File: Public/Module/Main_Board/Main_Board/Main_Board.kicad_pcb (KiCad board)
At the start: 2 copper layers, 4 parts, among them J1 Conn_02x28_Odd_Even, J2 Conn_02x28_Odd_Even, J3 Conn_02x28_Odd_Even, J4 Conn_02x28_Odd_Even

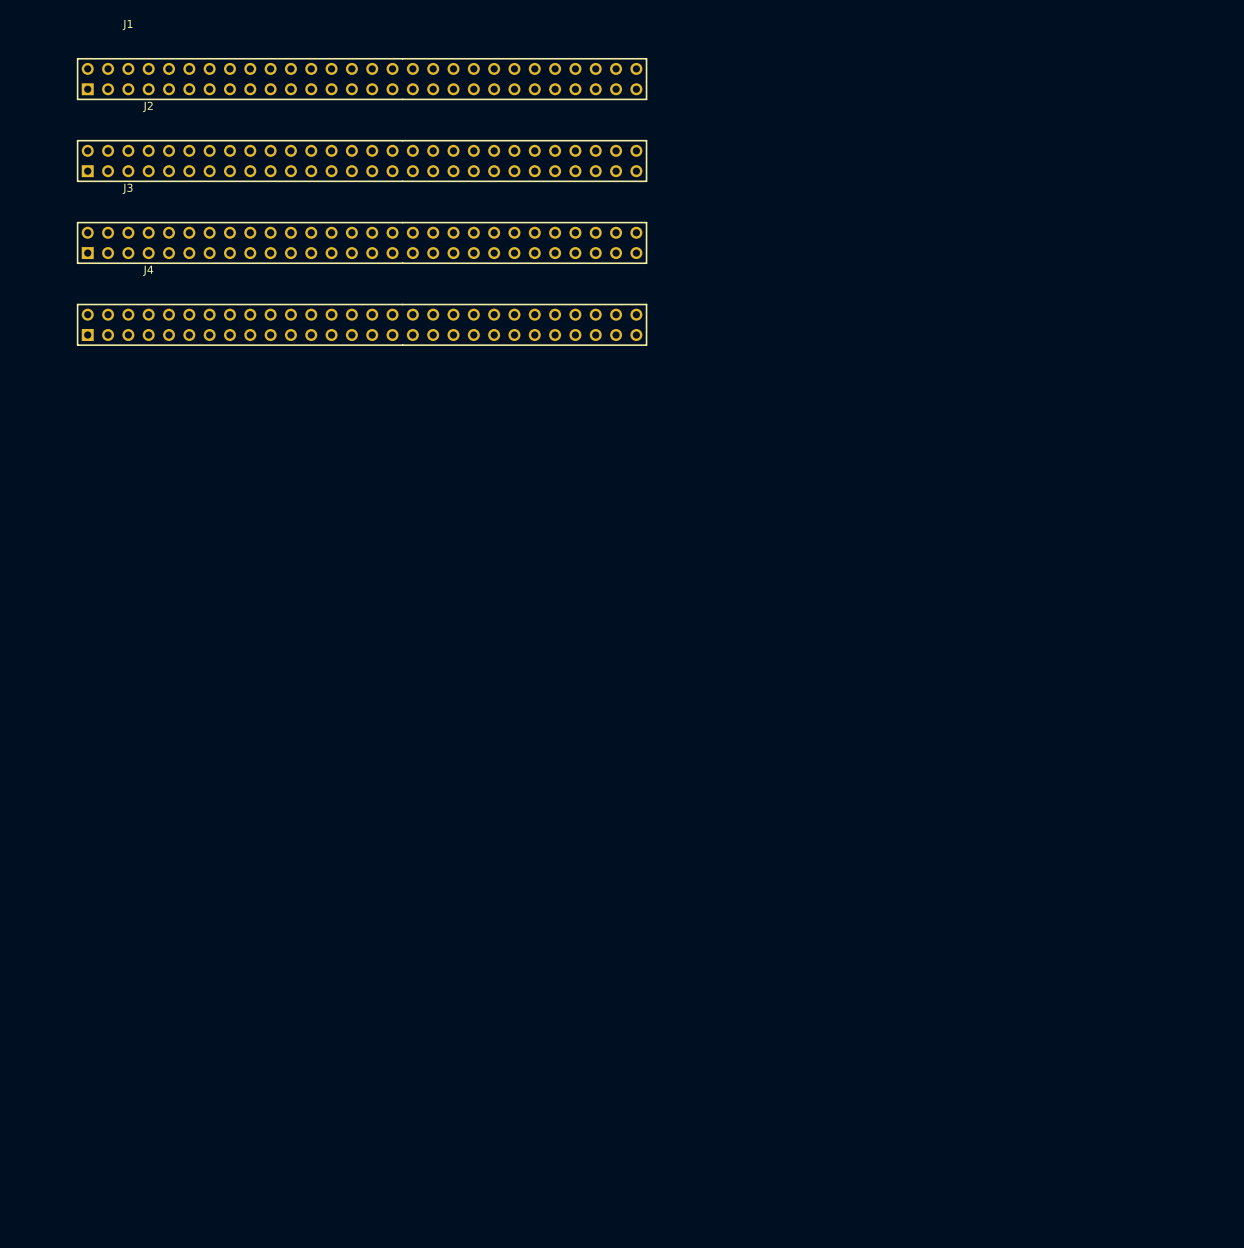
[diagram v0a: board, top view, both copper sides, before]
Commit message: 主板PCB绘制
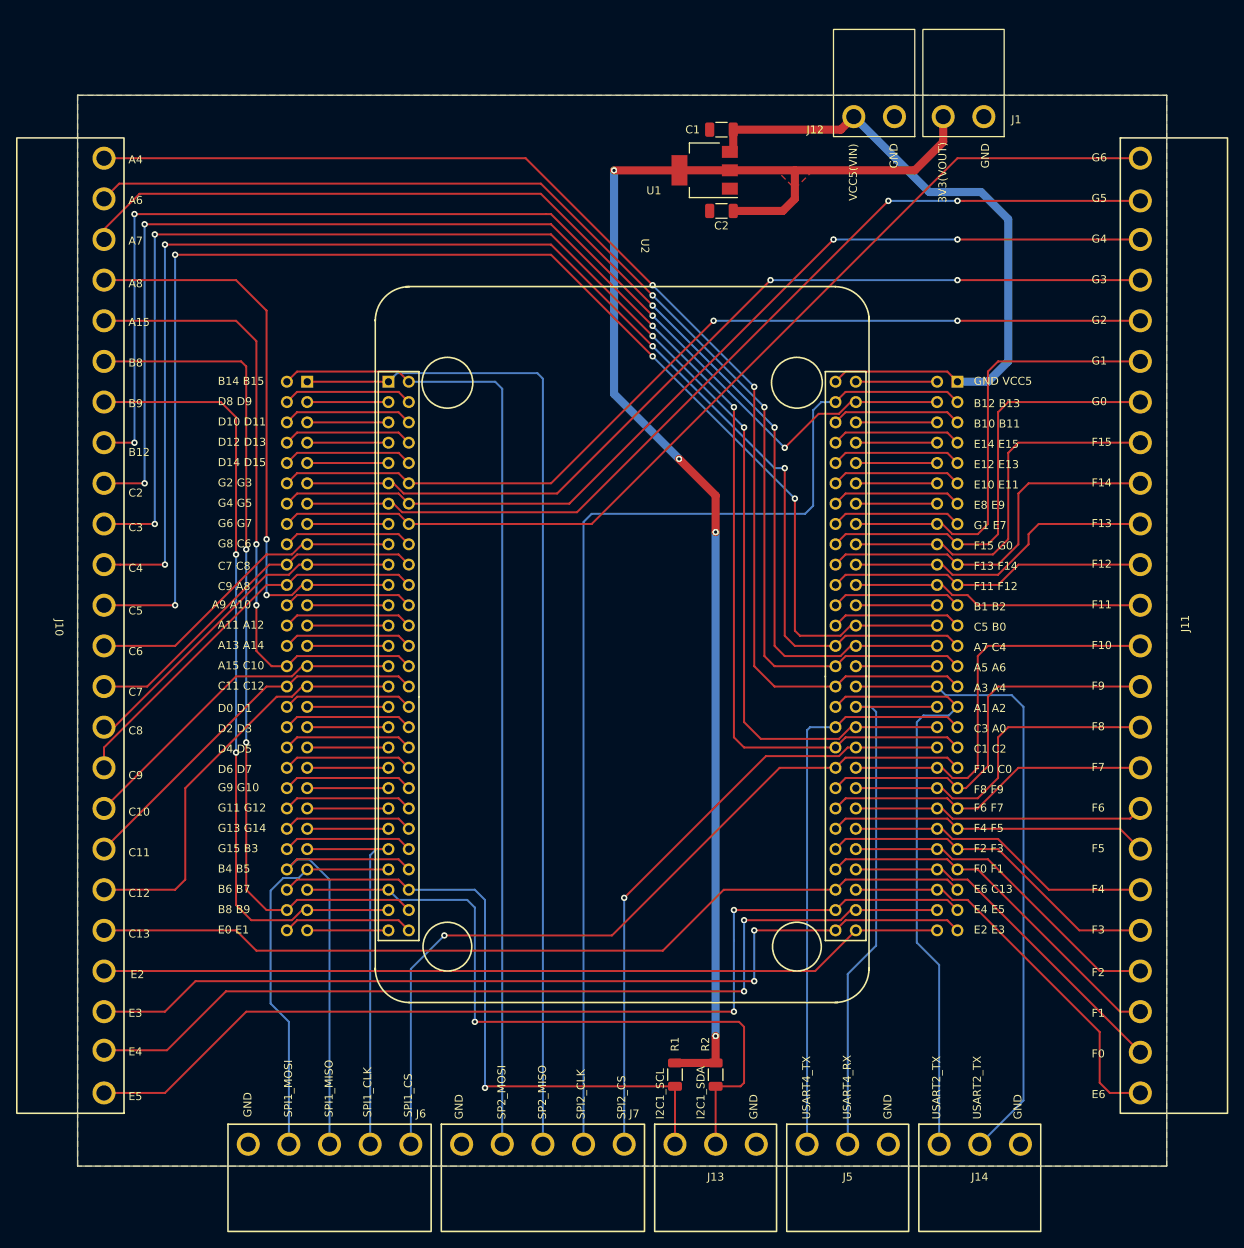
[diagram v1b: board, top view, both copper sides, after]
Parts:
- removed J2: Conn_02x28_Odd_Even, NEUDC:MCU_left
- added C1: 10uF, Capacitor_SMD:C_1206_3216Metric, F.Cu at (112.7, 42.1)
- added C2: 10uF, Capacitor_SMD:C_1206_3216Metric, F.Cu at (112.7, 52.3)
- added J10: Conn_01x24, NEUDC:Con_1_24, F.Cu at (35.6, 104.1)
- added J11: Conn_01x24, NEUDC:Con_1_24, F.Cu at (165.1, 104.1)
- added J12: Conn_01x02, NEUDC:Con_1_2, F.Cu at (131.8, 40.5)
- added J13: Conn_01x03, NEUDC:Con_1_3, F.Cu at (112.0, 169.0)
- added J14: Conn_01x03, NEUDC:Con_1_3, F.Cu at (145.0, 169.0)
- added J5: Conn_01x03, NEUDC:Con_1_3, F.Cu at (128.5, 169.0)
- added J6: Conn_01x05, NEUDC:Con_1_5, F.Cu at (63.8, 169.0)
- added J7: Conn_01x05, NEUDC:Con_1_5, F.Cu at (90.4, 169.0)
- added R1: 4.7k, Resistor_SMD:R_1206_3216Metric, F.Cu at (106.9, 160.3)
- added R2: 4.7k, Resistor_SMD:R_1206_3216Metric, F.Cu at (112.0, 160.3)
- added U1: LM1117MP-3.3, Package_TO_SOT_SMD:SOT-223-3_TabPin2, F.Cu at (110.6, 47.2)
- added U2: ~, NEUDC:qimin, F.Cu at (102.7, 56.7)
- J1: value Conn_02x28_Odd_Even -> Conn_01x02; footprint NEUDC:MCU_right -> NEUDC:Con_1_2
- J3, J4: moved to B.Cu
- moved J1 105.0 mm to (143.0, 40.5), turned to 180 degrees
- moved J3 100.2 mm to (134.6, 78.7), turned to -90 degrees
- moved J4 24.4 mm to (53.3, 81.3), turned to -90 degrees
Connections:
- J1 pad 1: /VCC5 -> GNDREF
- J1 pad 2: GNDREF -> /3V3
- J3 pad 3: /PB13 -> SPI2_CLK
- J3 pad 32: /PA3 -> USART2_RX
- J3 pad 33: /PA2 -> USART2_TX
- J3 pad 34: /PA1 -> USART4_RX
- J3 pad 35: /PA0 -> USART4_TX
- J3 pad 38: /PC1 -> SPI2_CS
- J3 pad 39: /PC0 -> SPI1_CS
- J4 pad 1: /PB14 -> SPI2_MISO
- J4 pad 2: /PB15 -> SPI2_MOSI
- J4 pad 47: /PB3 -> SPI1_CLK
- J4 pad 49: /PB5 -> SPI1_MOSI
- J4 pad 50: /PB4 -> SPI1_MISO
- J4 pad 51: /PB7 -> I2C1_SDA
- J4 pad 52: /PB6 -> I2C1_SCL
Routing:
- net /PC2: track 0.00 -> 191.4 mm, vias 0 -> 4
- net /PC3: track 0.00 -> 188.6 mm, vias 0 -> 4
- net /PC4: track 0.00 -> 180.8 mm, vias 0 -> 4
- net /3V3: track 0.00 -> 179.6 mm, vias 0 -> 4
- net /PC5: track 0.00 -> 177.9 mm, vias 0 -> 4
- net /PA4: track 0.00 -> 155.6 mm, vias 0 -> 2
- net /PA6: track 0.00 -> 151.7 mm, vias 0 -> 2
- net /PA7: track 0.00 -> 147.7 mm, vias 0 -> 2
- net /PB12: track 0.00 -> 147.2 mm, vias 0 -> 4
- net SPI2_CLK: track 0.00 -> 138.8 mm
- net /PG6: track 0.00 -> 126.7 mm
- net SPI2_MISO: track 0.00 -> 125.9 mm
- net /PE5: track 0.00 -> 124.7 mm, vias 0 -> 2
- net SPI2_MOSI: track 0.00 -> 122.8 mm
- net /PG4: track 0.00 -> 121.4 mm, vias 0 -> 2
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- added copper zone on F.Cu, net /3V3
- added copper zone on B.Cu, net GNDREF
- added copper zone on F.Cu, net GNDREF
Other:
- board outline added: 136.1 x 133.9 mm
- board text added: "3V3(VOUT)"
- board text added: "A1 A2"
- board text added: "A11 A12"
- board text added: "A13 A14"
- board text added: "A15"
- board text added: "A15 C10"
- board text added: "A3 A4"
- board text added: "A4"
- board text added: "A5 A6"
- board text added: "A6"
- board text added: "A7"
- board text added: "A7 C4"
- board text added: "A8"
- board text added: "A9 A10"
- board text added: "B1 B2"
- board text added: "B10 B11"
- board text added: "B12"
- board text added: "B12 B13"
- board text added: "B14 B15"
- board text added: "B4 B5"
- board text added: "B6 B7"
- board text added: "B8"
- board text added: "B8 B9"
- board text added: "B9"
- board text added: "C1 C2"
- board text added: "C10"
- board text added: "C11"
- board text added: "C11 C12"
- board text added: "C12"
- board text added: "C13"
- board text added: "C2"
- board text added: "C3"
- board text added: "C3 A0"
- board text added: "C4"
- board text added: "C5"
- board text added: "C5 B0"
- board text added: "C6"
- board text added: "C7"
- board text added: "C7 C8"
- board text added: "C8"
- board text added: "C9"
- board text added: "C9 A8"
- board text added: "D0 D1"
- board text added: "D10 D11"
- board text added: "D12 D13"
- board text added: "D14 D15"
- board text added: "D2 D3"
- board text added: "D4 D5"
- board text added: "D6 D7"
- board text added: "D8 D9"
- board text added: "E0 E1"
- board text added: "E10 E11"
- board text added: "E12 E13"
- board text added: "E14 E15"
- board text added: "E2"
- board text added: "E2 E3"
- board text added: "E3"
- board text added: "E4"
- board text added: "E4 E5"
- board text added: "E5"
- board text added: "E6"
- board text added: "E6 C13"
- board text added: "E8 E9"
- board text added: "F0"
- board text added: "F0 F1"
- board text added: "F1"
- board text added: "F10"
- board text added: "F10 C0"
- board text added: "F11"
- board text added: "F11 F12"
- board text added: "F12"
- board text added: "F13"
- board text added: "F13 F14"
- board text added: "F14"
- board text added: "F15"
- board text added: "F15 G0"
- board text added: "F2"
- board text added: "F2 F3"
- board text added: "F3"
- board text added: "F4"
- board text added: "F4 F5"
- board text added: "F5"
- board text added: "F6"
- board text added: "F6 F7"
- board text added: "F7"
- board text added: "F8"
- board text added: "F8 F9"
- board text added: "F9"
- board text added: "G0"
- board text added: "G1"
- board text added: "G1 E7"
- board text added: "G11 G12"
- board text added: "G13 G14"
- board text added: "G15 B3"
- board text added: "G2"
- board text added: "G2 G3"
- board text added: "G3"
- board text added: "G4"
- board text added: "G4 G5"
- board text added: "G5"
- board text added: "G6"
- board text added: "G6 G7"
- board text added: "G8 C6"
- board text added: "G9 G10"
- board text added: "GND"
- board text added: "GND VCC5"
- board text added: "I2C1_SCL"
- board text added: "I2C1_SDA"
- board text added: "SP2_MISO"
- board text added: "SP2_MOSI"
- board text added: "SPI1_CLK"
- board text added: "SPI1_CS"
- board text added: "SPI1_MISO"
- board text added: "SPI1_MOSI"
- board text added: "SPI2_CLK"
- board text added: "SPI2_CS"
- board text added: "USART2_TX"
- board text added: "USART4_RX"
- board text added: "USART4_TX"
- board text added: "VCC5(VIN)"
